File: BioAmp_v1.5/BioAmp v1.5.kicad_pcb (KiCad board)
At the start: 2 copper layers, 32 x 60 mm, 33 parts, among them J1 Conn_01x02_Male, J2 PJ-3062-CO, J4 Conn_01x03_Male, J5 Conn_01x02_Male, J6 Conn_01x02_Male, J7 Conn_01x02_Male, U1 TL074

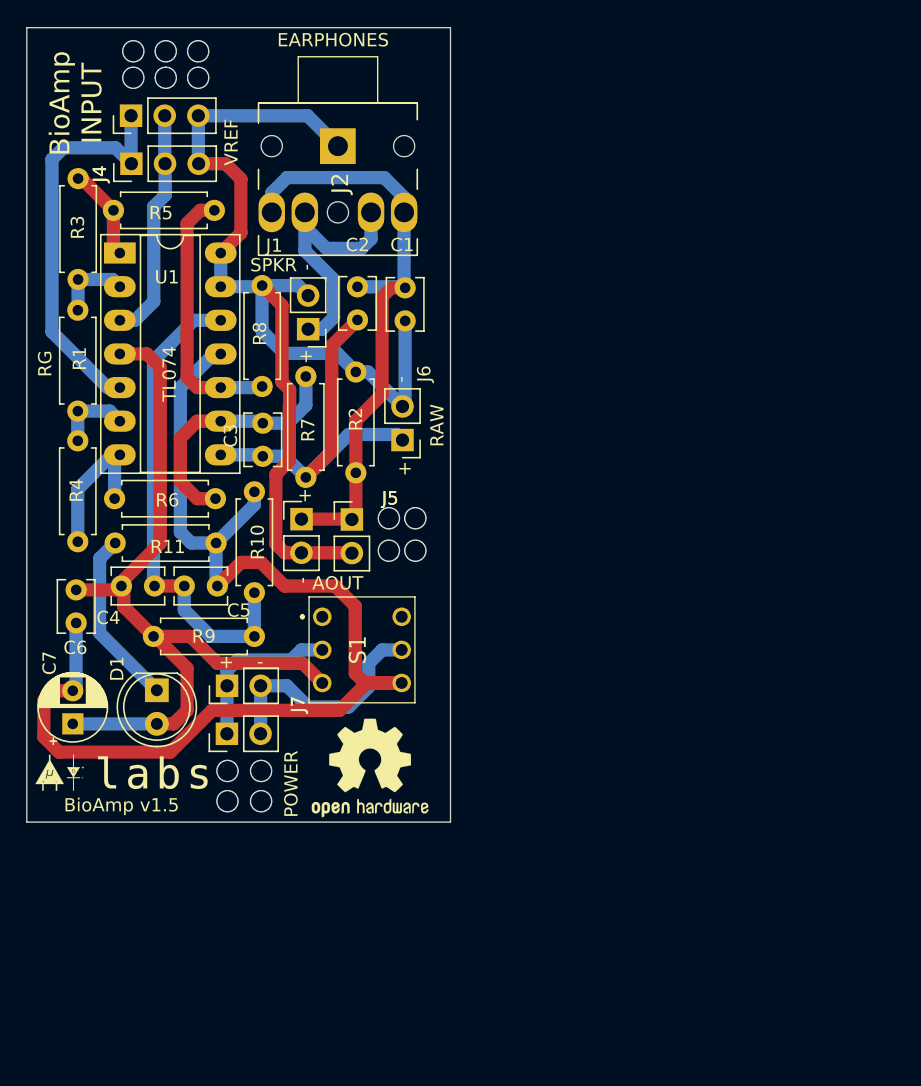
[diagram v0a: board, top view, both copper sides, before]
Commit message: update v1.5.4
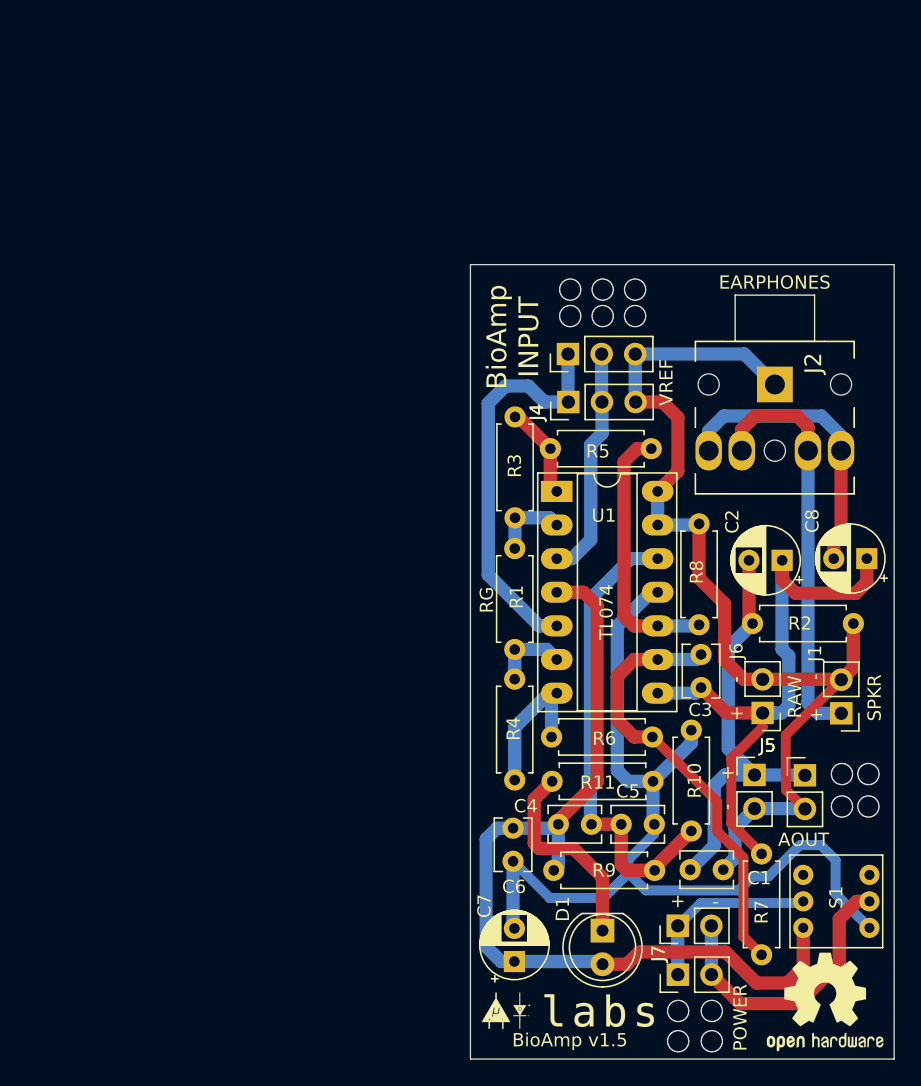
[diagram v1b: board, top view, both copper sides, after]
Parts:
- removed the REF** at (115.9, 103.9) (x2)
- added C8: CP, Capacitor_THT:CP_Radial_D5.0mm_P2.50mm, F.Cu at (153.4, 88.1)
- added REF**: OSHW-Logo2_9.8x8mm_SilkScreen, Symbol:OSHW-Logo2_9.8x8mm_SilkScreen, F.Cu at (150.3, 121.6)
- added REF**: OSHW-Logo2_9.8x8mm_SilkScreen, Symbol:OSHW-Logo2_9.8x8mm_SilkScreen, B.Cu at (150.3, 121.6)
- C2: value 100nf -> CP; footprint Capacitor_THT:C_Disc_D3.8mm_W2.6mm_P2.50mm -> Capacitor_THT:CP_Radial_D5.0mm_P2.50mm
- S1: footprint udlabs:TL2285EE -> udlabs:G64_DPDT
- moved R7 55.6 mm to (145.5, 118.0), turned to 90 degrees
- moved J1 49.6 mm to (151.5, 99.8)
- moved C1 47.9 mm to (142.6, 111.6), turned to 180 degrees
- moved S1 39.7 mm to (151.6, 111.0)
- moved J5 39.3 mm to (148.8, 104.5)
- moved J5 39.3 mm to (145.0, 104.4)
- moved J7 38.6 mm to (139.2, 119.5)
- moved J7 38.6 mm to (139.2, 115.8)
- moved D1 38.2 mm to (133.5, 116.2)
- moved G*** 38.2 mm to (130.9, 122.2)
- moved C2 38.1 mm to (147.0, 88.2), turned to 180 degrees
- moved C7 37.9 mm to (126.8, 118.5)
- moved C4 37.6 mm to (132.6, 108.2)
- moved R11 37.6 mm to (129.7, 104.9)
- moved C5 37.6 mm to (137.4, 108.2)
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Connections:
- C2 pad 1: ACout -> Aout
- C2 pad 2: Aout -> ACout
- J2 pad 2: ACout -> ACout_spkr
- J2 pad 3: ACout -> ACout_spkr
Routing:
- net ACout_spkr: track 0.00 -> 22.1 mm
- net GND: track 88.0 -> 70.9 mm
- net Aout: track 29.5 -> 46.2 mm
- net ACout: track 46.6 -> 32.2 mm
- net Net-(C3-Pad1): track 20.0 -> 34.1 mm
- net Net-(J1-Pad1): track 20.2 -> 31.1 mm
- net +9V: track 59.9 -> 68.6 mm
- net Vref: track 84.3 -> 77.4 mm
- net B-: track 17.8 -> 21.6 mm
- net Net-(D1-Pad1): track 13.4 -> 15.5 mm
- net Net-(C4-Pad1): track 37.5 -> 36.1 mm
- net B+: track 12.6 -> 13.9 mm
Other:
- board text added: "AUXOUT"
- board text added: "S"
